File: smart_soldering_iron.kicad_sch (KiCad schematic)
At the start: 20 parts, among them U1 ATMEGA328PB-AU

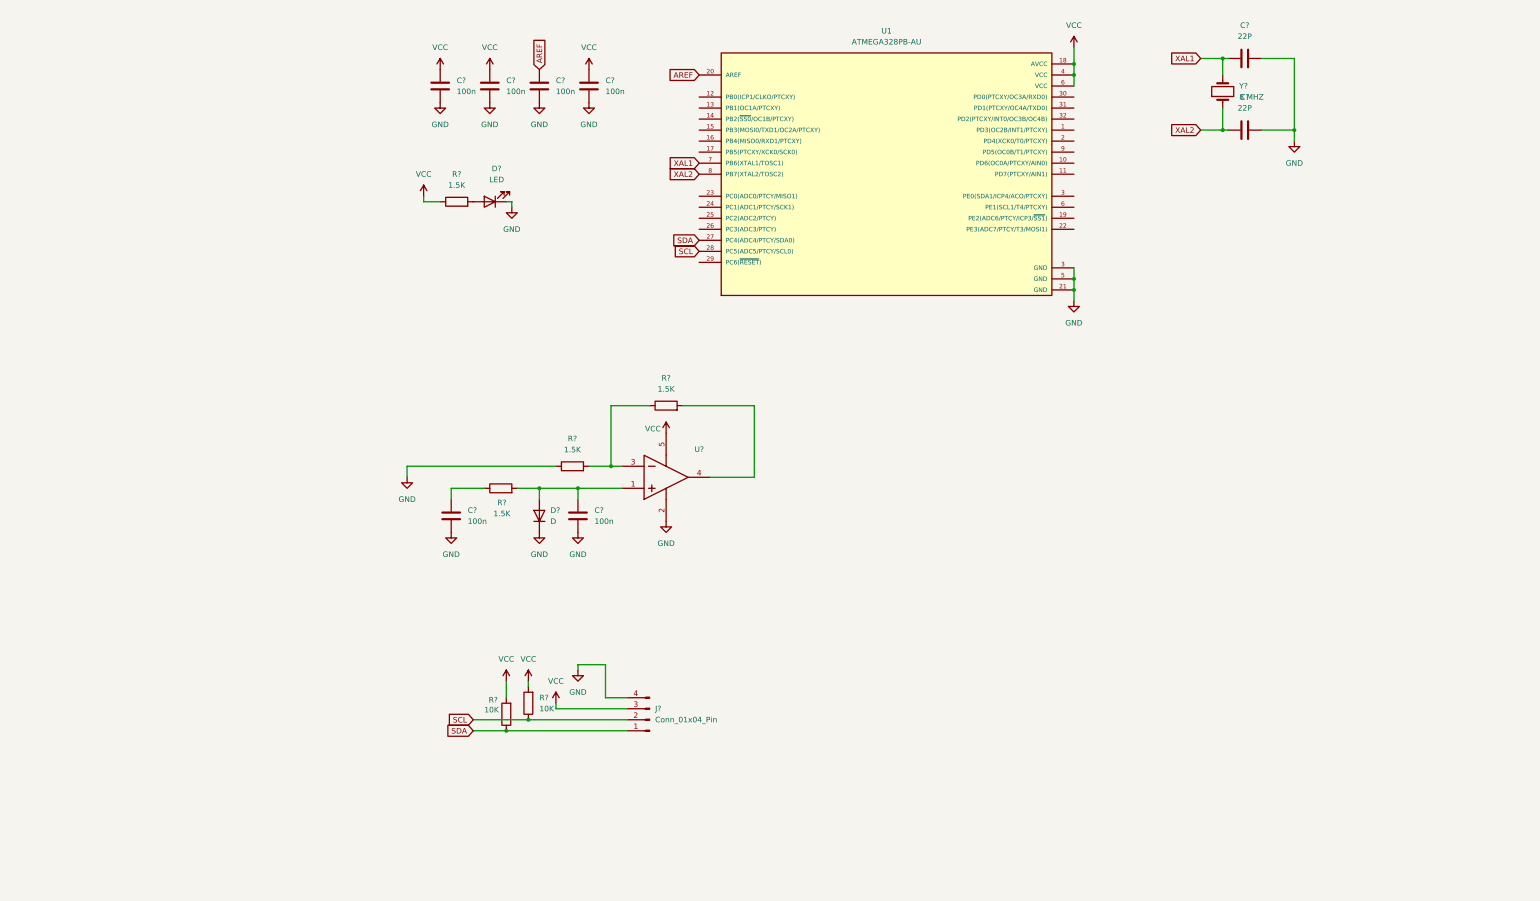
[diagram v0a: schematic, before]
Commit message: test
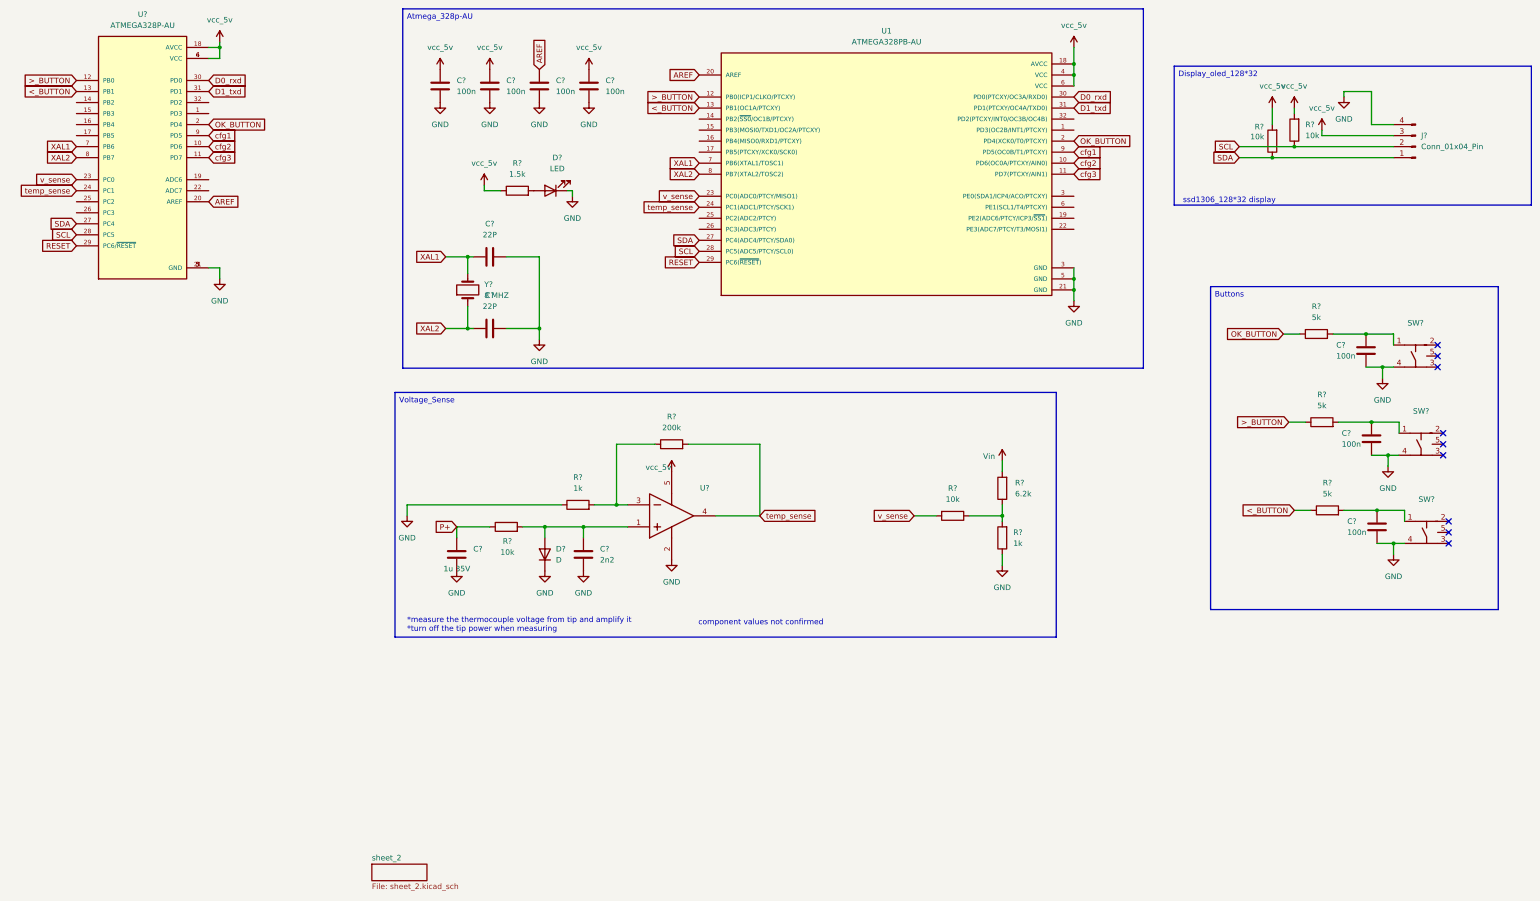
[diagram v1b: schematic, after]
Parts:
- added C? (x3): 100n, symbol Device:C
- added R? (x3): 5k, symbol Device:R
- added R?: 10k, symbol Device:R
- added R?: 6.2k, symbol Device:R
- added R?: 1k, symbol Device:R
- added SW? (x3): ~, ProLib_pcs_2025-10-04:SW-SMD_4P-L3.4-W3.4-P2.00-LS4.0_TS3315A160GF, symbol smart_soldering_iron:GT-TC028B-H0070-L1
- added U?: ATMEGA328P-AU, ATMEGA328P-AU:QFP80P900X900X120-32N, symbol smart_soldering_iron:ATMEGA328P-AU
- C?: value 100n -> 1u 35V
- C?: value 100n -> 2n2
- R?: value 1.5K -> 10k
- R?: value 1.5K -> 200k
- R? (x2): value 10K -> 10k
- R?: value 1.5K -> 1k
- R?: value 1.5K -> 1.5k
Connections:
- net VCC is gone; now on net vcc_5v: C?.1, C?.1, C?.1, J?.3 (Pin_3), R?.1, R?.2, R?.2, U1.18 (AVCC), U1.4 (VCC), U1.6 (VCC), U?.5 (V+)
- net AREF: now also U?.20 (AREF)
- net GND: now also C?.1, C?.1, C?.1, R?.1, SW?.4, SW?.4, SW?.4, U?.21 (GND), U?.3 (GND), U?.5 (GND)
- net SCL: now also U?.28 (PC5)
- net SDA: now also U?.27 (PC4)
- net XAL1: now also U?.7 (PB6)
- net XAL2: now also U?.8 (PB7)
- net P+: now reaches C?.1, R?.1
- net cfg2: now reaches U1.10 (PD6(OC0A/PTCXY/AIN0))
- net cfg2: now also U?.10 (PD6)
- net cfg3: now reaches U1.11 (PD7(PTCXY/AIN1))
- net cfg3: now also U?.11 (PD7)
- net >_BUTTON: now reaches U1.12 (PB0(ICP1/CLKO/PTCXY))
- net >_BUTTON: now also R?.1, U?.12 (PB0)
- net <_BUTTON: now reaches U1.13 (PB1(OC1A/PTCXY))
- net <_BUTTON: now also R?.1, U?.13 (PB1)
- net OK_BUTTON: now reaches U1.2 (PD4(XCK0/T0/PTCXY))
- net OK_BUTTON: now also R?.1, U?.2 (PD4)
- net v_sense: now reaches U1.23 (PC0(ADC0/PTCY/MISO1))
- net v_sense: now also R?.2, U?.23 (PC0)
- net temp_sense: now reaches U1.24 (PC1(ADC1/PTCY/SCK1))
- net temp_sense: now also R?.2, U?.4 (OUT), U?.24 (PC1)
- net RESET: now reaches U1.29 (PC6(~{RESET}))
- net RESET: now also U?.29 (PC6/~{RESET})
- net D0_rxd: now reaches U1.30 (PD0(PTCXY/OC3A/RXD0))
- net D0_rxd: now also U?.30 (PD0)
- net D1_txd: now reaches U1.31 (PD1(PTCXY/OC4A/TXD0))
- net D1_txd: now also U?.31 (PD1)
- net vcc_5v: now reaches U1.6 (VCC)
- net vcc_5v: now also U?.18 (AVCC), U?.4 (VCC), U?.6 (VCC)
- net cfg1: now reaches U1.9 (PD5(OC0B/T1/PTCXY))
- net cfg1: now also U?.9 (PD5)
- new net: C?.2, R?.2, SW?.1 (x3)
- new net: R?.1, R?.1, R?.2
- new net Vin: R?.2
- no-connect marks 0 -> 9
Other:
- added sheet sheet_2 (sheet_2.kicad_sch)
- note added: "*measure the thermocouple voltage from tip and amplify it *turn off the tip power when measuring"
- note added: "component values not confirmed"
- note added: "ssd1306_128*32 display"
- moved on the sheet: C?, D?, J?, R?, U?, Y?
